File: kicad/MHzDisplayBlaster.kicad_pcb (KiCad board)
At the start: 2 copper layers, 39.6 x 31.2 mm, 5 parts, among them J1 Conn_02x15 DigitRHS, J2 Conn_02x15 DigitLHS, J4 Conn_01x07, U1 DC56-11GWA

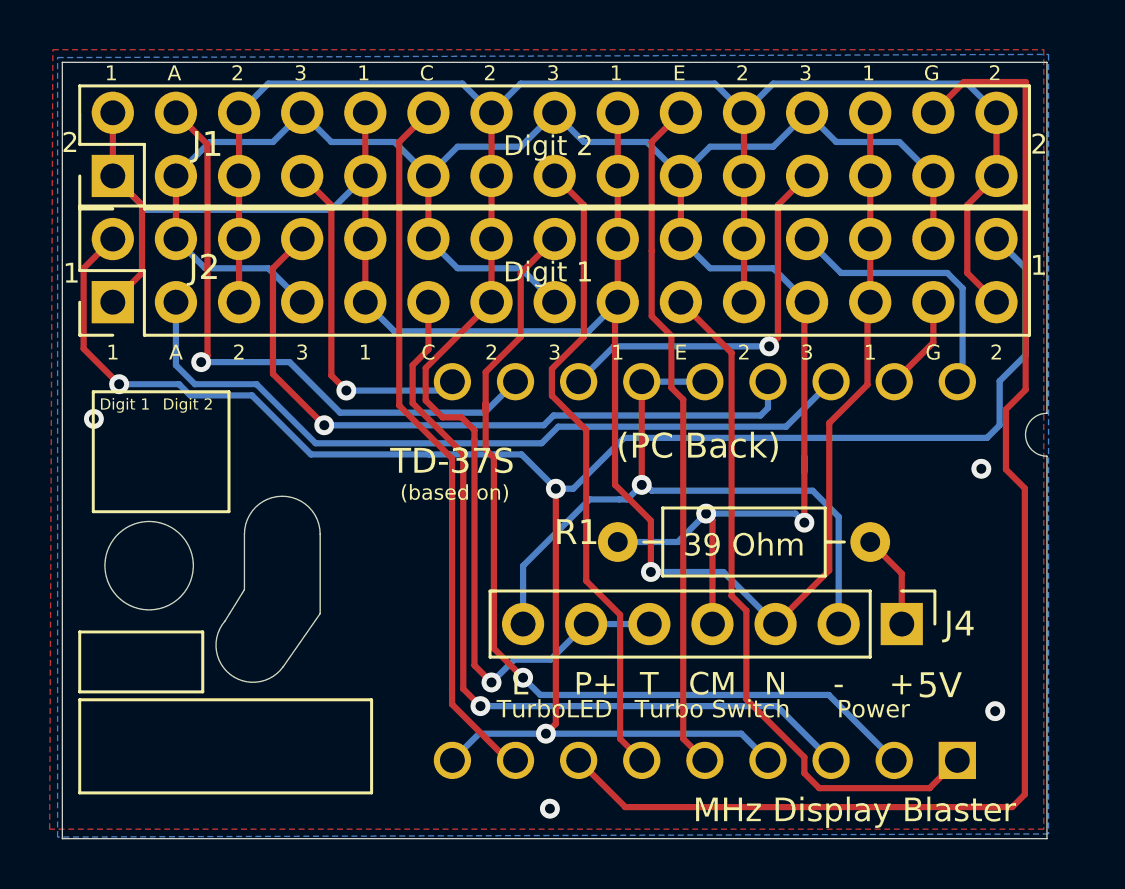
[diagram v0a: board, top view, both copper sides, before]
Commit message: Update KICAD version
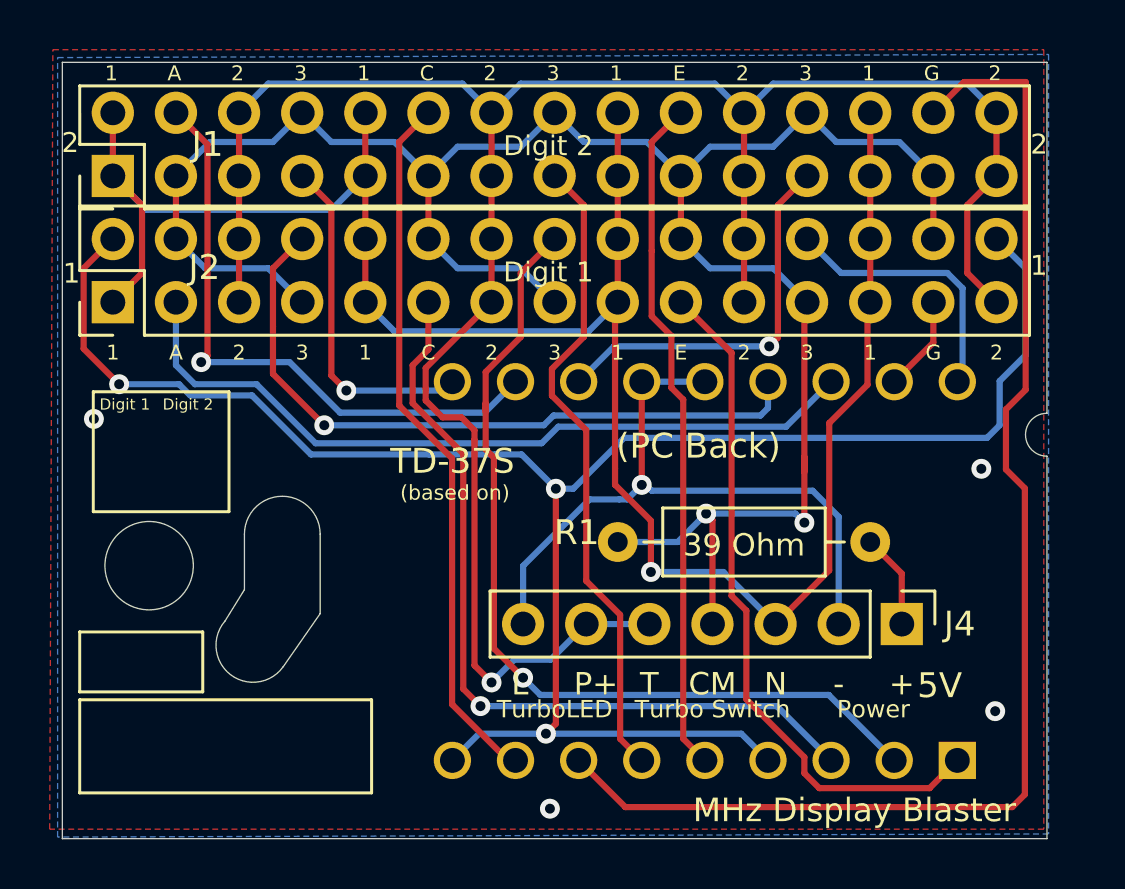
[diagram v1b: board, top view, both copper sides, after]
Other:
- net class Default removed
